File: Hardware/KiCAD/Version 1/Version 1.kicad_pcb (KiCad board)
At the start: 2 copper layers, 95 x 98 mm, 6 parts

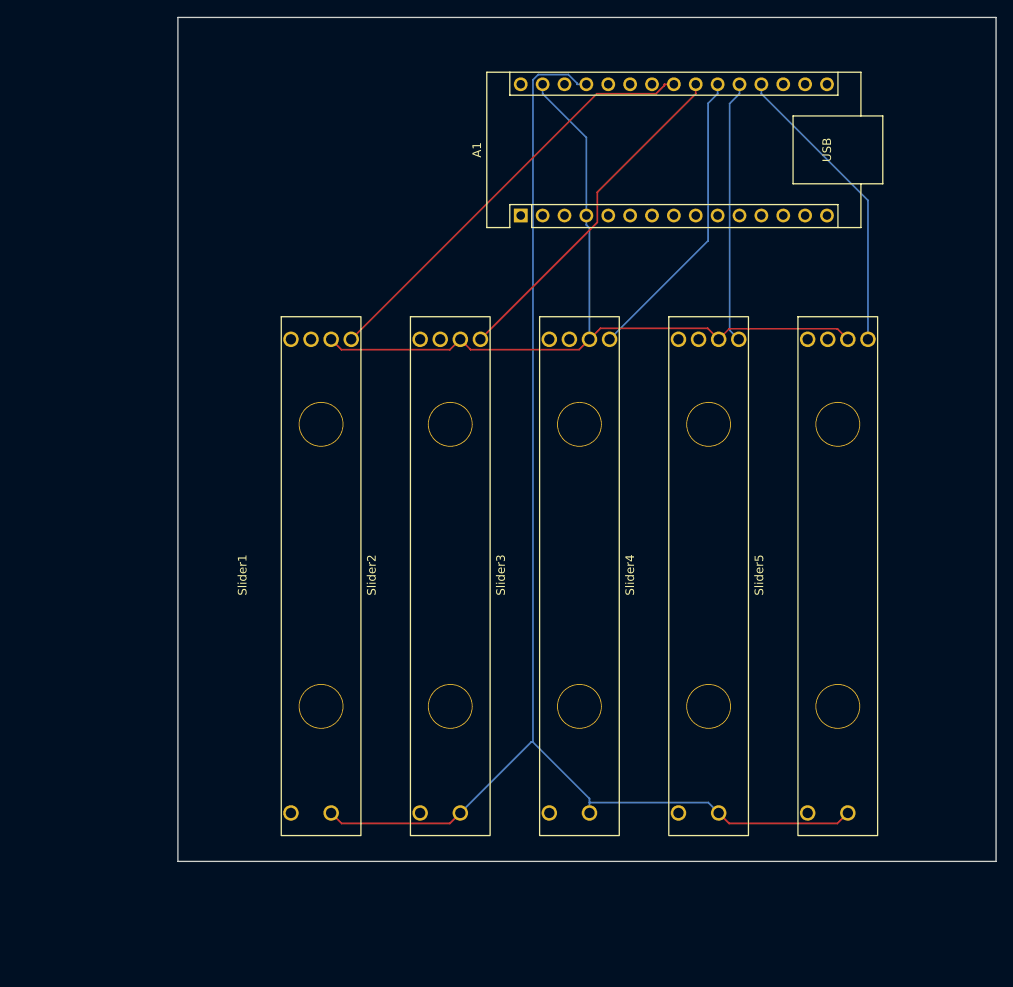
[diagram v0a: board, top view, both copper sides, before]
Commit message: pcb progress
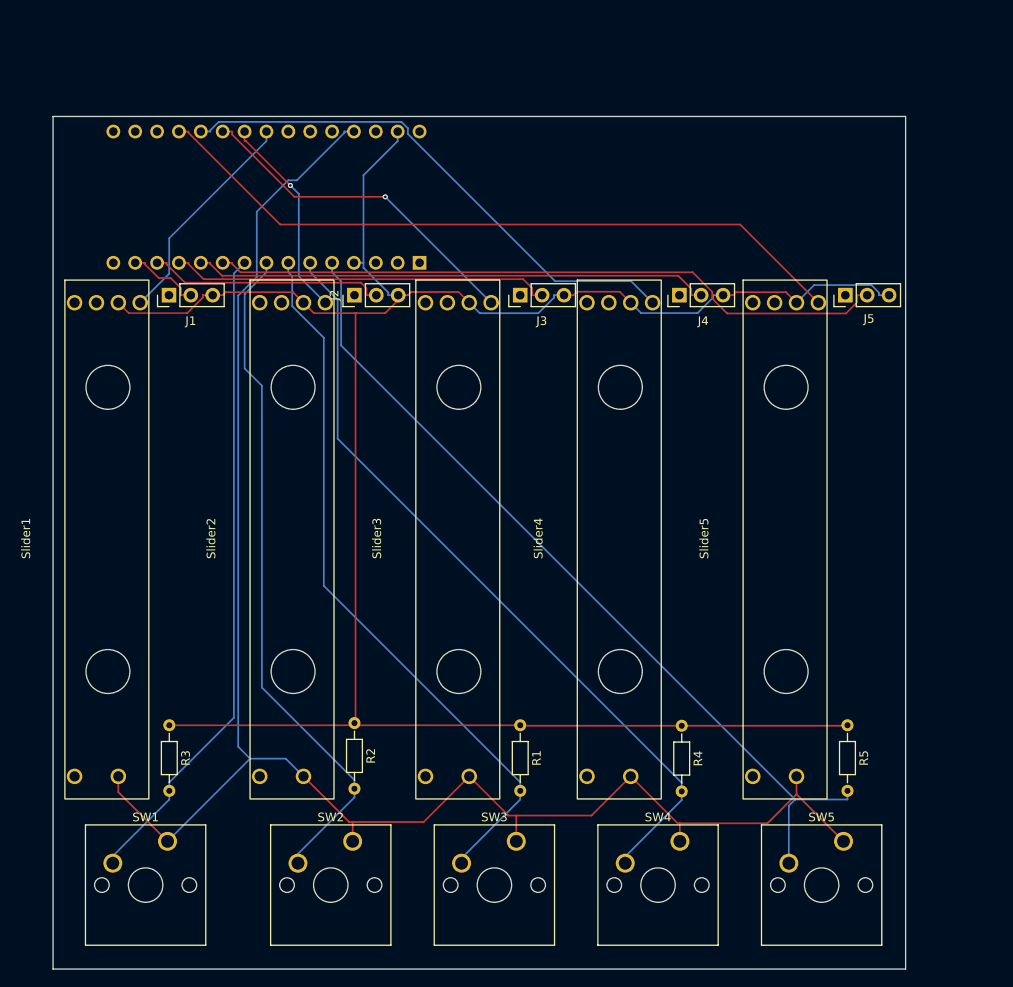
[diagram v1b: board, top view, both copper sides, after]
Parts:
- added J1: Conn_01x03_Pin, Connector_PinHeader_2.54mm:PinHeader_1x03_P2.54mm_Vertical, F.Cu at (62.0, 65.0)
- added J2: Conn_01x03_Pin, Connector_PinHeader_2.54mm:PinHeader_1x03_P2.54mm_Vertical, F.Cu at (83.5, 65.0)
- added J3: Conn_01x03_Pin, Connector_PinHeader_2.54mm:PinHeader_1x03_P2.54mm_Vertical, F.Cu at (102.8, 65.0)
- added J4: Conn_01x03_Pin, Connector_PinHeader_2.54mm:PinHeader_1x03_P2.54mm_Vertical, F.Cu at (121.2, 65.0)
- added J5: Conn_01x03_Pin, Connector_PinHeader_2.54mm:PinHeader_1x03_P2.54mm_Vertical, F.Cu at (140.5, 65.0)
- added R1: 10K, Resistor_THT:R_Axial_DIN0204_L3.6mm_D1.6mm_P7.62mm_Horizontal, F.Cu at (102.8, 114.9)
- added R2: 10K, Resistor_THT:R_Axial_DIN0204_L3.6mm_D1.6mm_P7.62mm_Horizontal, F.Cu at (83.5, 114.7)
- added R3: 10K, Resistor_THT:R_Axial_DIN0204_L3.6mm_D1.6mm_P7.62mm_Horizontal, F.Cu at (62.0, 114.9)
- added R4: 10K, Resistor_THT:R_Axial_DIN0204_L3.6mm_D1.6mm_P7.62mm_Horizontal, F.Cu at (121.5, 115.0)
- added R5: 10K, Resistor_THT:R_Axial_DIN0204_L3.6mm_D1.6mm_P7.62mm_Horizontal, F.Cu at (140.8, 114.9)
- added SW1: Button 1, Button_Switch_Keyboard:SW_Cherry_MX_1.00u_PCB, F.Cu at (61.8, 128.4)
- added SW2: Button 2, Button_Switch_Keyboard:SW_Cherry_MX_1.00u_PCB, F.Cu at (83.3, 128.4)
- added SW3: Button 3, Button_Switch_Keyboard:SW_Cherry_MX_1.00u_PCB, F.Cu at (102.3, 128.4)
- added SW4: Button 4, Button_Switch_Keyboard:SW_Cherry_MX_1.00u_PCB, F.Cu at (121.3, 128.4)
- added SW5: Button 5, Button_Switch_Keyboard:SW_Cherry_MX_1.00u_PCB, F.Cu at (140.3, 128.4)
- A1: moved to B.Cu
- moved Slider1 25.5 mm to (49.9, 63.2)
- moved Slider2 19.1 mm to (71.4, 63.2)
- moved Slider3 15.0 mm to (90.6, 63.2)
- moved A1 13.0 mm to (91.1, 61.2)
- moved Slider4 11.4 mm to (109.4, 63.2)
- moved Slider5 7.66 mm to (128.6, 63.2)
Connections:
- A1 pad 10: unconnected-(A1-D7-Pad10) -> Net-(A1-D7)
- A1 pad 11: unconnected-(A1-D8-Pad11) -> Net-(A1-D8)
- A1 pad 12: unconnected-(A1-D9-Pad12) -> Net-(A1-D9)
- A1 pad 13: unconnected-(A1-D10-Pad13) -> Net-(A1-D10)
- A1 pad 14: unconnected-(A1-MOSI-Pad14) -> Net-(A1-MOSI)
- A1 pad 5: unconnected-(A1-D2-Pad5) -> Net-(A1-D2)
- A1 pad 6: unconnected-(A1-D3-Pad6) -> Net-(A1-D3)
- A1 pad 7: unconnected-(A1-D4-Pad7) -> Net-(A1-D4)
- A1 pad 8: unconnected-(A1-D5-Pad8) -> Net-(A1-D5)
- A1 pad 9: unconnected-(A1-D6-Pad9) -> Net-(A1-D6)
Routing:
- net GND: track 95.9 -> 250.9 mm
- net Net-(A1-D2): track 0.00 -> 99.4 mm
- net Net-(A1-D3): track 0.00 -> 90.3 mm
- net Net-(A1-D4): track 0.00 -> 83.7 mm
- net Net-(A1-D7): track 0.00 -> 79.2 mm
- net Net-(A1-D5): track 0.00 -> 78.8 mm
- net Net-(A1-D6): track 0.00 -> 76.1 mm
- net Net-(A1-D8): track 0.00 -> 60.2 mm
- net Net-(A1-A0): track 34.7 -> 82.6 mm
- net Net-(A1-D9): track 0.00 -> 44.3 mm
- net +5V: track 154.2 -> 196.9 mm
- net Net-(A1-A1): track 30.5 -> 62.1 mm
- net Net-(A1-D10): track 0.00 -> 27.6 mm
- net Net-(A1-SDA/A4): track 49.8 -> 25.9 mm
- net Net-(A1-A3): track 40.0 -> 23.9 mm, vias 0 -> 1
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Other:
- board size 95 x 98 mm -> 99 x 99 mm
